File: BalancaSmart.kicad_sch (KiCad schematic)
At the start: 49 parts, among them J1 Load Cell, Q3 NMOS, Q4 S8050, Q5 IRF7309PBF, SW1 SW_Push, U1 HX711-Mod, U2 ADS1115-module, U3 HX-2S-JH20, U4 XL4015

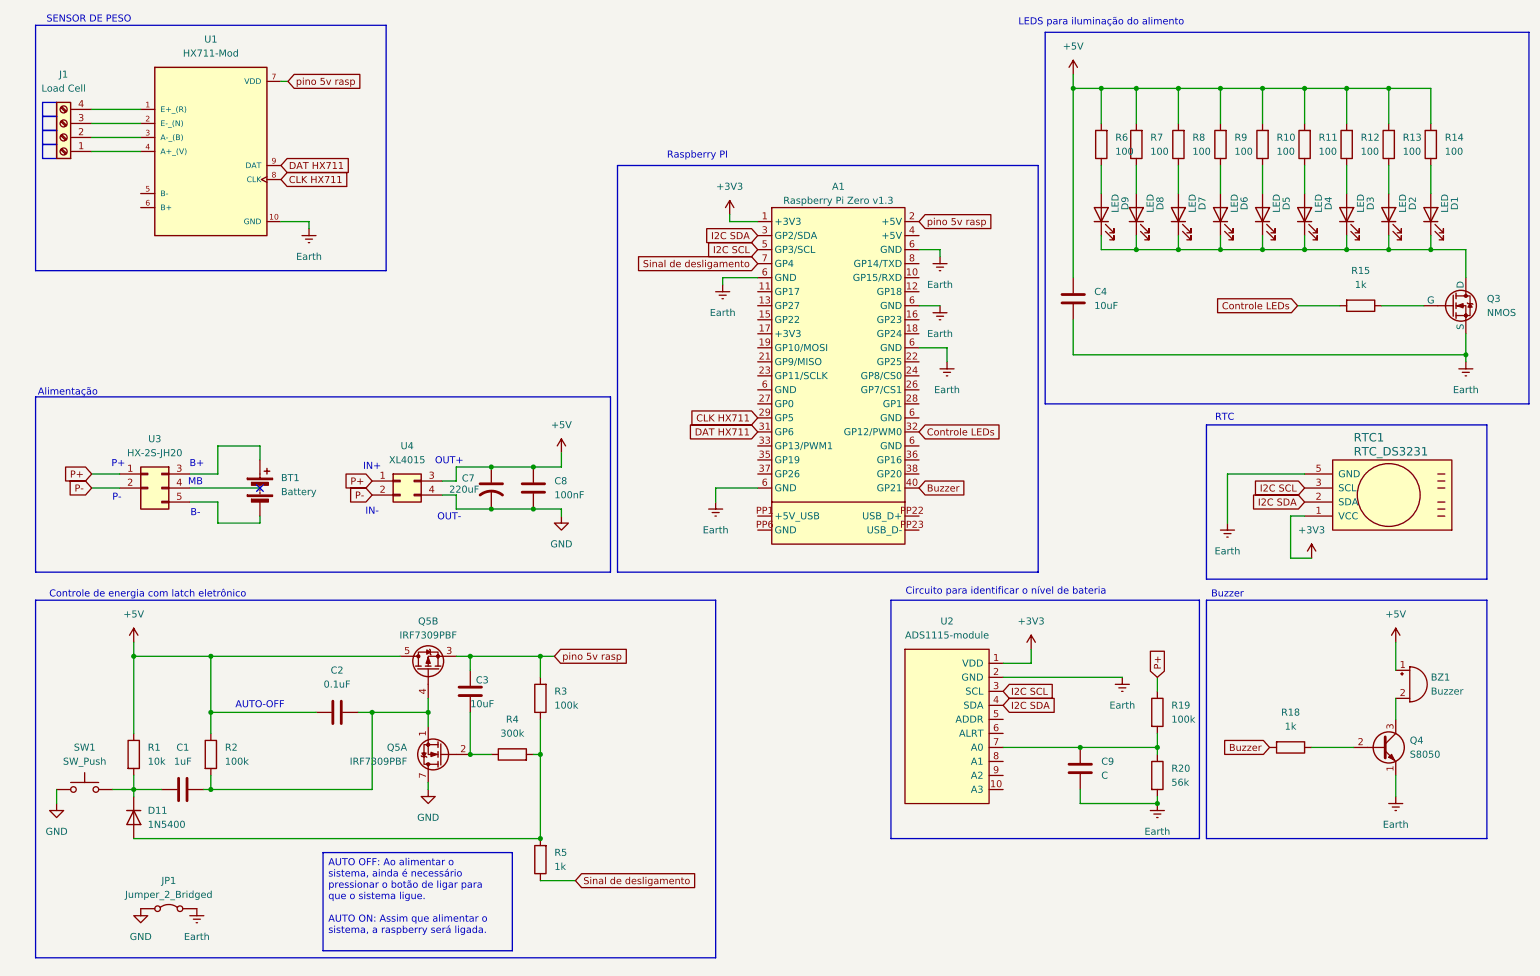
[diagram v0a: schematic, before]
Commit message: alterações no circuito
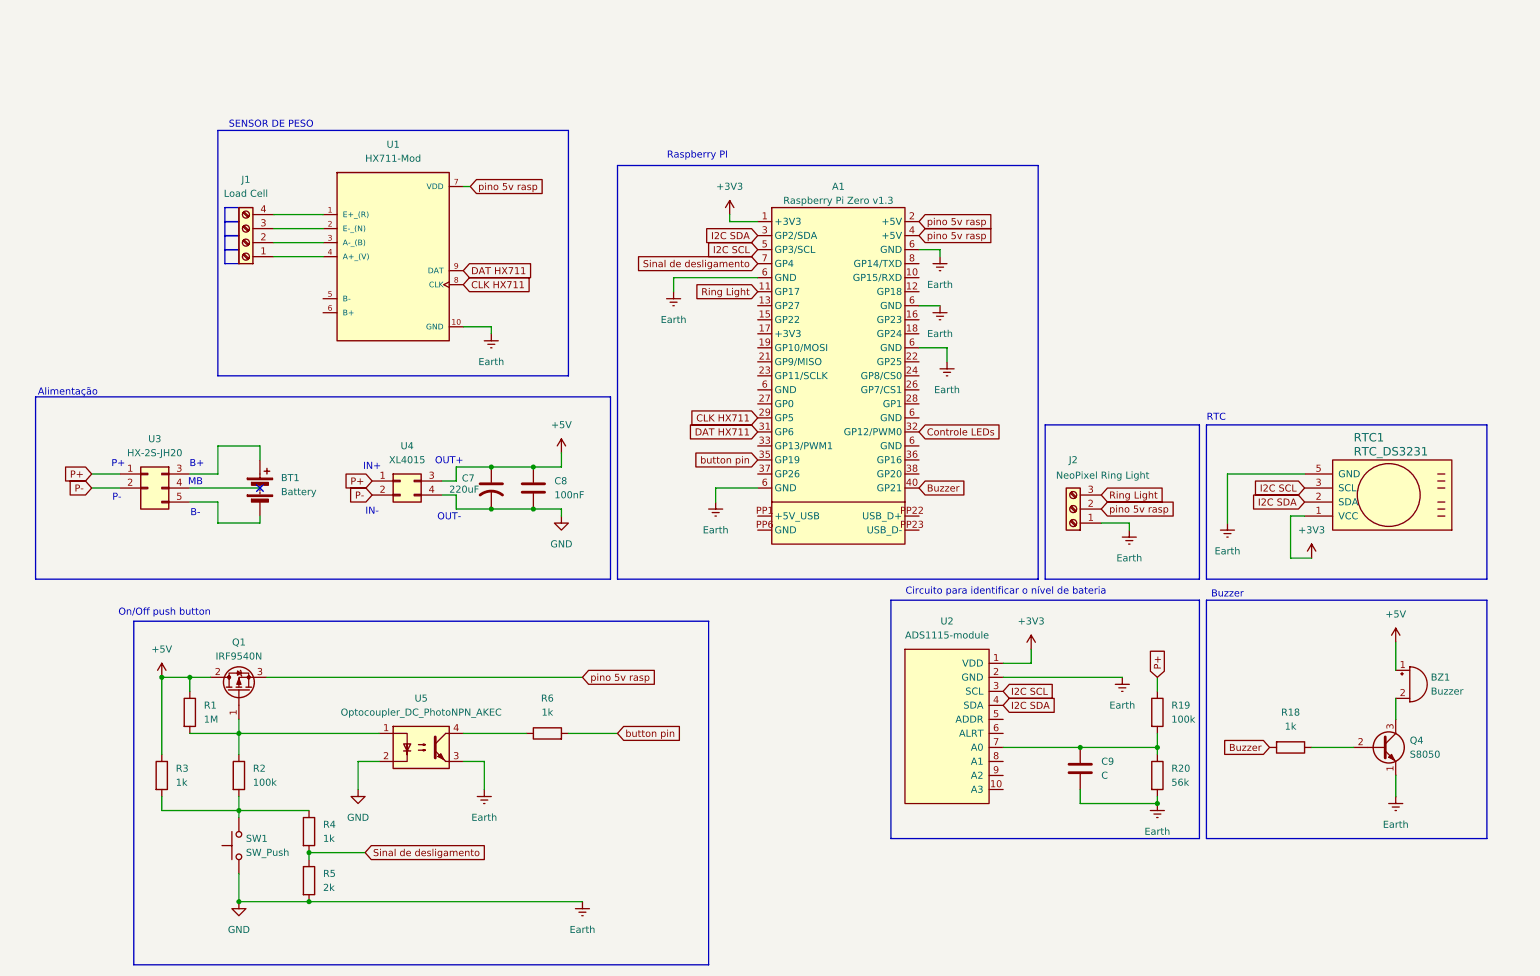
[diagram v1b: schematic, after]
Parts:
- removed C1: 1uF, Capacitor_THT:C_Disc_D5.0mm_W2.5mm_P2.50mm, symbol Device:C
- removed C2: 0.1uF, Capacitor_THT:C_Disc_D5.0mm_W2.5mm_P2.50mm, symbol Device:C
- removed C3: 10uF, Capacitor_THT:C_Disc_D5.0mm_W2.5mm_P2.50mm, symbol Device:C
- removed C4: 10uF, Capacitor_THT:C_Radial_D6.3mm_H7.0mm_P2.50mm, symbol Device:C
- removed D1, D2, D3, D4, D5, D6, D7, D8, D9: LED, Connector_PinHeader_2.54mm:PinHeader_1x02_P2.54mm_Vertical, symbol Device:LED
- removed D11: 1N5400, Diode_THT:D_DO-201AD_P15.24mm_Horizontal, symbol Diode:1N5400
- removed JP1: Jumper_2_Bridged, Resistor_THT:R_Axial_DIN0204_L3.6mm_D1.6mm_P7.62mm_Horizontal, symbol Jumper:Jumper_2_Bridged
- removed Q3: NMOS, Package_TO_SOT_THT:TO-220-3_Vertical, symbol Simulation_SPICE:NMOS
- removed Q5: IRF7309PBF, Package_SO:SOIC-8_3.9x4.9mm_P1.27mm, symbol Transistor_FET:IRF7309PBF
- removed R10, R11, R12, R13, R14, R7, R8, R9: 100, Resistor_THT:R_Axial_DIN0204_L3.6mm_D1.6mm_P7.62mm_Horizontal, symbol Device:R
- removed R15: 1k, Resistor_THT:R_Axial_DIN0204_L3.6mm_D1.6mm_P7.62mm_Horizontal, symbol Device:R
- added J2: NeoPixel Ring Light, symbol Connector:Screw_Terminal_01x03
- added Q1: IRF9540N, Package_TO_SOT_THT:TO-220-3_Vertical, symbol Transistor_FET:IRF9540N
- added U5: Optocoupler_DC_PhotoNPN_AKEC, symbol Isolator:Optocoupler_DC_PhotoNPN_AKEC
- BT1, SW1: footprint TerminalBlock:TerminalBlock_MaiXu_MX126-5.0-02P_1x02_P5.00mm -> (none)
- R1: value 10k -> 1M; footprint Resistor_THT:R_Axial_DIN0204_L3.6mm_D1.6mm_P7.62mm_Horizontal -> (none)
- R2: footprint Resistor_THT:R_Axial_DIN0204_L3.6mm_D1.6mm_P7.62mm_Horizontal -> (none)
- R3: value 100k -> 1k; footprint Resistor_THT:R_Axial_DIN0204_L3.6mm_D1.6mm_P7.62mm_Horizontal -> (none)
- R4: value 300k -> 1k; footprint Resistor_THT:R_Axial_DIN0204_L3.6mm_D1.6mm_P7.62mm_Horizontal -> (none)
- R5: value 1k -> 2k; footprint Resistor_THT:R_Axial_DIN0204_L3.6mm_D1.6mm_P7.62mm_Horizontal -> (none)
- R6: value 100 -> 1k; footprint Resistor_THT:R_Axial_DIN0204_L3.6mm_D1.6mm_P7.62mm_Horizontal -> (none)
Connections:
- net GND is gone; now on net Earth: C7.2, C8.2, SW1.1, U4.4 (Pin_4)
- net +5V: now also R3.1, Q1.2 (D); no longer R2.1, R6.2
- net Earth: now also R5.2, J2.1 (Pin_1), U5.2, U5.3
- net Sinal de desligamento: now also R4.2
- net pino 5v rasp: now also A1.4 (+5V), J2.2 (Pin_2), Q1.3 (S); no longer R3.2
- net at SW1.2: now also R2.2, R3.2, R4.1; no longer R1.2
- net Ring Light: now reaches A1.11 (GP17)
- net Ring Light: now also J2.3 (Pin_3)
- net button pin: now reaches A1.35 (GP19)
- net button pin: now also R6.2
- net at R6.1: now also U5.4
- new net: Q1.1 (G), R1.2, R2.1, U5.1
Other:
- note added: "On/Off push button"
- note removed: "AUTO-OFF"
- note removed: "Controle de energia com latch eletrônico"
- note removed: "LEDS para iluminação do alimento"
- moved on the sheet: J1, U1

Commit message: organização do esquemático
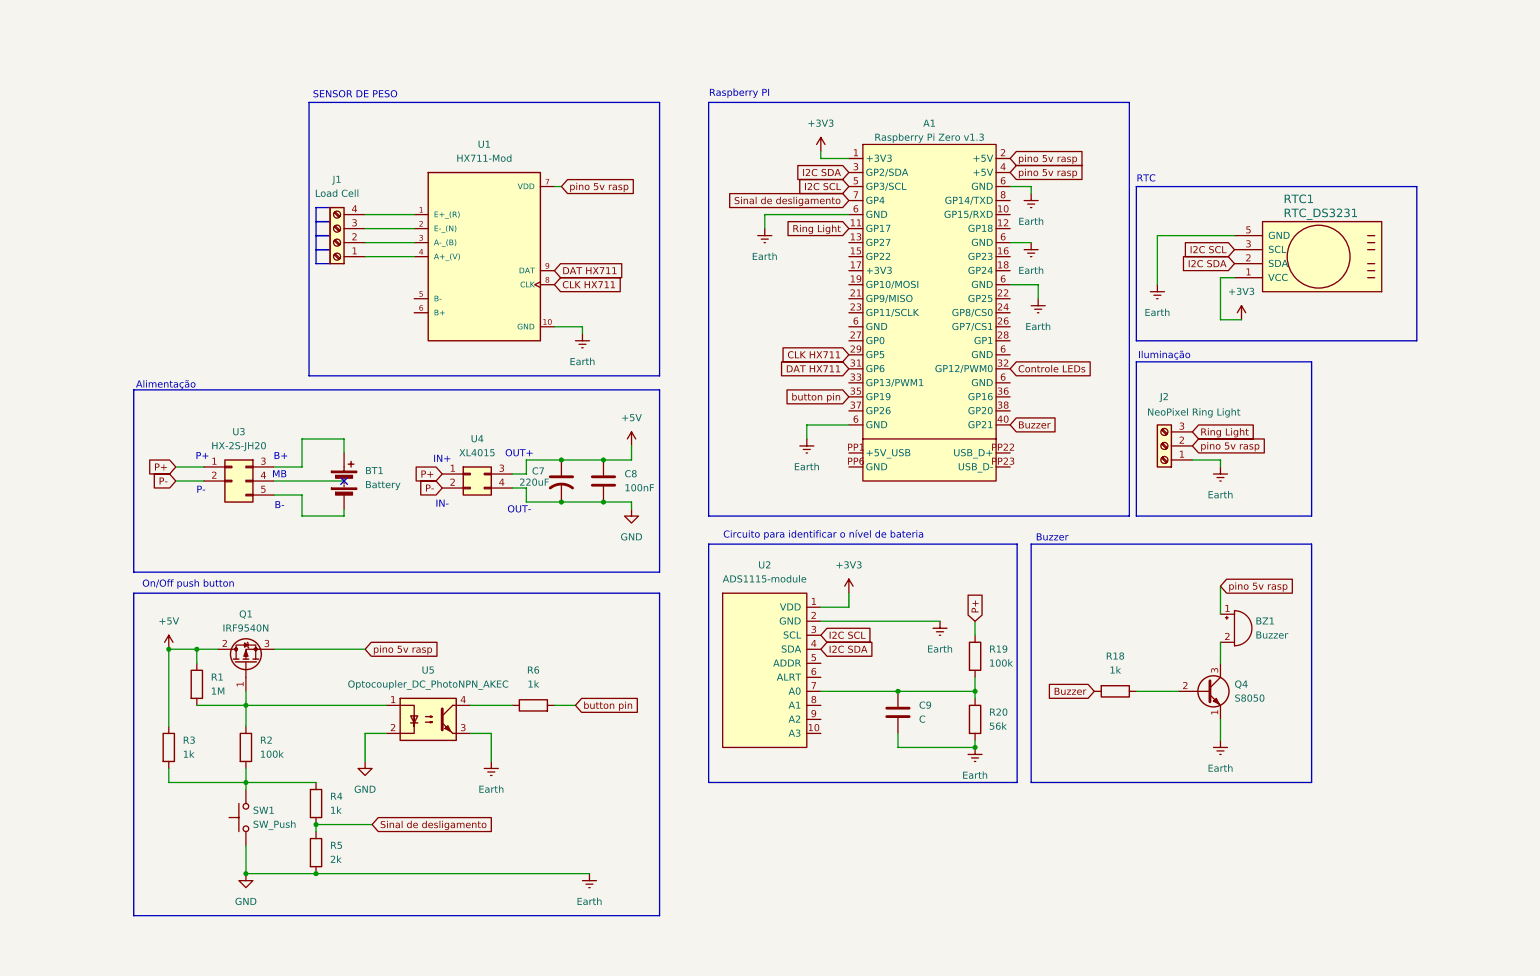
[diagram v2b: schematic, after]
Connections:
- net +5V: no longer BZ1.1 (+)
- net pino 5v rasp: now also BZ1.1 (+)
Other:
- note added: "Iluminação"
- moved on the sheet: A1, BT1, BZ1, C7, C8, C9, J1, J2, Q1, Q4, R1, R18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

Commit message: trilhas
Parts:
- J2: footprint (none) -> TerminalBlock:TerminalBlock_MaiXu_MX126-5.0-03P_1x03_P5.00mm
- R1, R2, R3, R4, R5, R6: footprint (none) -> Resistor_THT:R_Axial_DIN0204_L3.6mm_D1.6mm_P7.62mm_Horizontal
- SW1: footprint (none) -> TerminalBlock:TerminalBlock_MaiXu_MX126-5.0-02P_1x02_P5.00mm
- U3: footprint TerminalBlock:TerminalBlock_MaiXu_MX126-5.0-04P_1x04_P5.00mm -> TerminalBlock:TerminalBlock_MaiXu_MX126-5.0-02P_1x02_P5.00mm
- U5: footprint (none) -> Package_DIP:DIP-4_W7.62mm_Socket_LongPads
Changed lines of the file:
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@@
 			)
 		)
-		(property "Footprint" ""
+		(property "Footprint" "Resistor_THT:R_Axial_DIN0204_L3.6mm_D1.6mm_P7.62mm_Horizontal"
 			(at 35.052 147.32 90)
 			(hide yes)
@@
 			)
 		)
-		(property "Footprint" ""
+		(property "Footprint" "TerminalBlock:TerminalBlock_MaiXu_MX126-5.0-03P_1x03_P5.00mm"
 			(at 217.17 92.71 0)
 			(hide yes)
@@
 			)
 		)
-		(property "Footprint" "TerminalBlock:TerminalBlock_MaiXu_MX126-5.0-04P_1x04_P5.00mm"
+		(property "Footprint" "TerminalBlock:TerminalBlock_MaiXu_MX126-5.0-02P_1x02_P5.00mm"
 			(at 50.8 99.06 0)
 			(hide yes)
@@
 			)
 		)
-		(property "Footprint" ""
+		(property "Footprint" "Resistor_THT:R_Axial_DIN0204_L3.6mm_D1.6mm_P7.62mm_Horizontal"
 			(at 61.722 157.48 90)
 			(hide yes)
@@
 			)
 		)
-		(property "Footprint" ""
+		(property "Footprint" "Resistor_THT:R_Axial_DIN0204_L3.6mm_D1.6mm_P7.62mm_Horizontal"
 			(at 102.87 141.478 90)
 			(hide yes)
@@
 			)
 		)
-		(property "Footprint" ""
+		(property "Footprint" "Resistor_THT:R_Axial_DIN0204_L3.6mm_D1.6mm_P7.62mm_Horizontal"
 			(at 40.132 135.89 90)
 			(hide yes)
@@
 			)
 		)
-		(property "Footprint" ""
+		(property "Footprint" "TerminalBlock:TerminalBlock_MaiXu_MX126-5.0-02P_1x02_P5.00mm"
 			(at 45.72 160.02 0)
 			(hide yes)
@@
 			)
 		)
-		(property "Footprint" ""
+		(property "Footprint" "Resistor_THT:R_Axial_DIN0204_L3.6mm_D1.6mm_P7.62mm_Horizontal"
 			(at 49.022 147.32 90)
 			(hide yes)
@@
 			)
 		)
-		(property "Footprint" ""
+		(property "Footprint" "Resistor_THT:R_Axial_DIN0204_L3.6mm_D1.6mm_P7.62mm_Horizontal"
 			(at 61.722 166.37 90)
 			(hide yes)
@@
 			)
 		)
-		(property "Footprint" ""
+		(property "Footprint" "Package_DIP:DIP-4_W7.62mm_Socket_LongPads"
 			(at 78.74 147.32 0)
 			(hide yes)
